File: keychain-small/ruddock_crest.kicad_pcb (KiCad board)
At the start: 2 copper layers, 38 x 45.3 mm, 4 parts

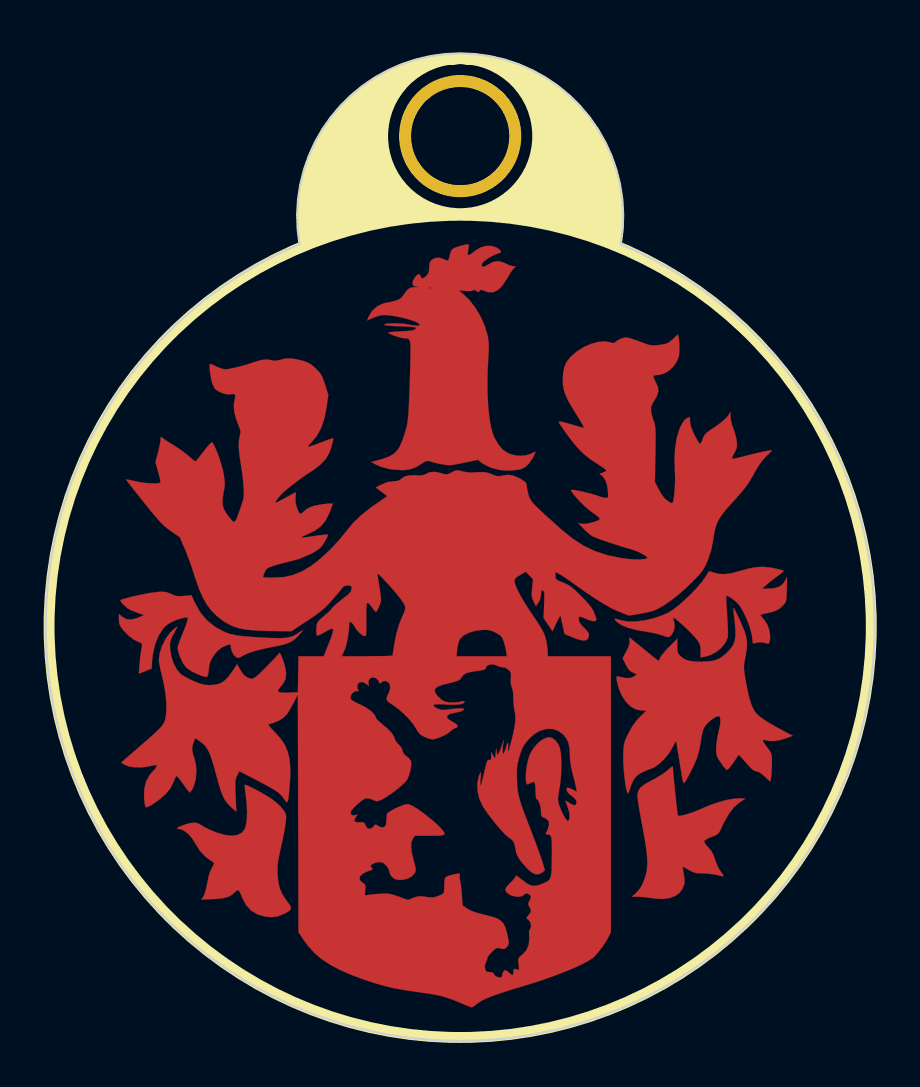
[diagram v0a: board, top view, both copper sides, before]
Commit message: New hole design
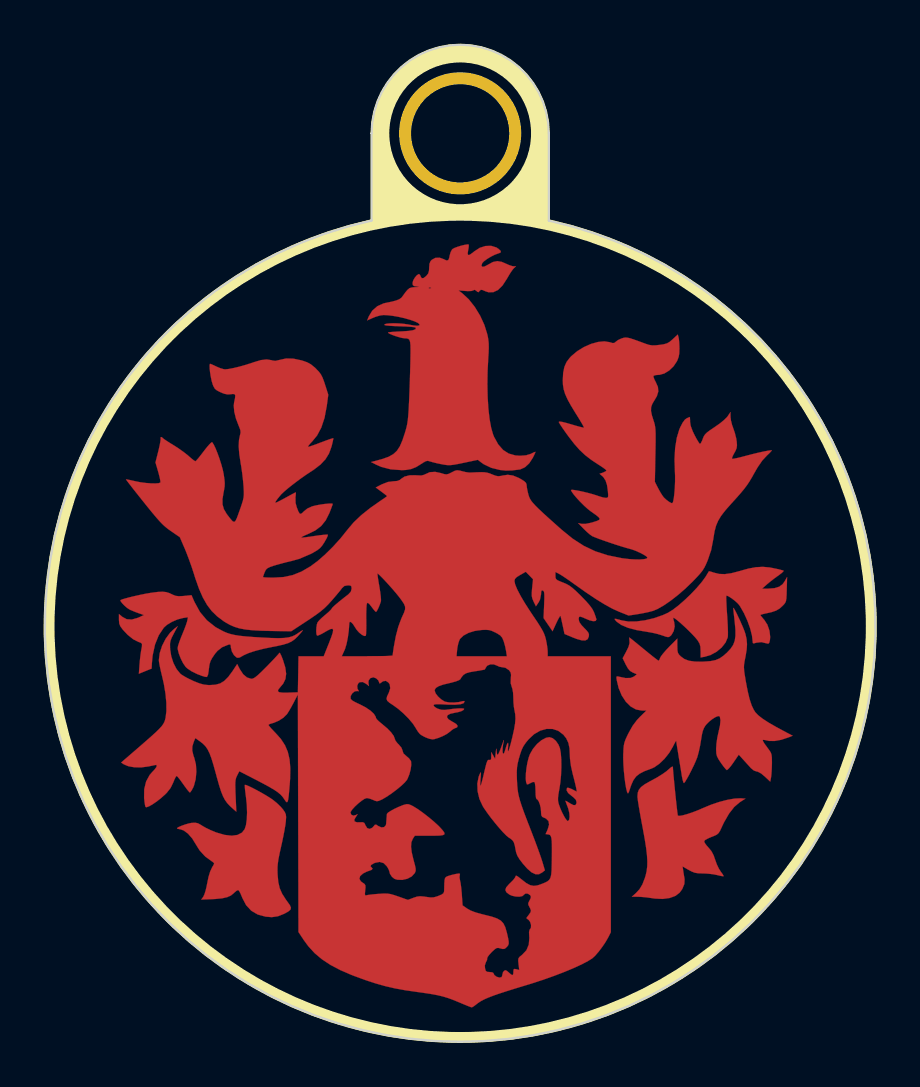
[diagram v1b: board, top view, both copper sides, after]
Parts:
- moved REF** 0.13 mm to (141.0, 85.3)
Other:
- board size 38 x 45.3 mm -> 38.1 x 45.7 mm
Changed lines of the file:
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@@
   (general
     (thickness 1.6)
-    (drawings 22)
+    (drawings 28)
     (tracks 0)
     (zones 0)
@@
   (title_block
     (title "Ruddock House PCB Crest")
-    (date 2019-02-12)
+    (date 2019-02-13)
     (rev A)
     (company "Ruddock House Electrical Engineering")
@@
   )
   (module MountingHole:MountingHole_3.2mm_M3_DIN965_Pad (layer F.Cu)
-    (at 140.97 85.471)
+    (at 140.97 85.344)
     (descr "Mounting Hole 3.2mm, M3, DIN965")
     (tags "mounting hole 3.2mm m3 din965")
@@
       (xy 9.730745 -13.40817) (xy 9.745385 -13.421618) (xy 9.978417 -13.636419) (xy 10.013345 -13.51111)) (layer F.Mask) (width 0.01))
   )
-  (dimension 41.529 (width 0.3) (layer Dwgs.User)
-    (gr_text "41.529 mm" (at 166.946 106.2355 270) (layer Dwgs.User)
+  (gr_poly (pts (xy 144.78 89.408) (xy 141.478 88.9) (xy 143.51 87.884) (xy 144.78 86.106)) (layer B.SilkS) (width 0.15))
+  (gr_poly (pts (xy 144.78 89.408) (xy 141.478 88.9) (xy 143.51 87.884) (xy 144.78 86.106)) (layer F.SilkS) (width 0.15))
+  (gr_poly (pts (xy 137.16 89.408) (xy 140.208 88.9) (xy 138.684 88.138) (xy 137.16 86.106)) (layer B.SilkS) (width 0.15))
+  (gr_poly (pts (xy 137.16 89.408) (xy 140.208 88.9) (xy 138.684 88.138) (xy 137.16 86.106)) (layer F.SilkS) (width 0.15))
+  (gr_line (start 137.16 85.344) (end 137.16 89.408) (layer B.SilkS) (width 0.57))
+  (gr_line (start 144.78 85.344) (end 144.78 89.408) (layer B.SilkS) (width 0.57))
+  (gr_line (start 144.78 85.344) (end 144.78 89.408) (layer F.SilkS) (width 0.57))
+  (gr_arc (start 140.97 85.344) (end 144.78 85.344) (angle -180) (layer B.SilkS) (width 0.57))
+  (gr_circle (center 140.97 85.344) (end 144.47 85.344) (layer B.SilkS) (width 0.5))
+  (gr_line (start 137.16 85.344) (end 137.16 89.408) (layer F.SilkS) (width 0.57))
+  (gr_arc (start 140.97 85.344) (end 144.78 85.344) (angle -180) (layer F.SilkS) (width 0.57))
+  (gr_line (start 145.034 85.344) (end 145.034 89.3445) (layer Edge.Cuts) (width 0.1))
+  (gr_line (start 136.906 85.344) (end 136.906 89.3445) (layer Edge.Cuts) (width 0.1))
+  (gr_arc (start 140.97 107.95) (end 136.906001 89.344501) (angle -335.3568188) (layer Edge.Cuts) (width 0.1))
+  (gr_line (start 121.92 107.95) (end 160.02 107.95) (layer Dwgs.User) (width 0.1))
+  (gr_arc (start 140.97 85.344) (end 145.034 85.344) (angle -180) (layer Edge.Cuts) (width 0.1))
+  (gr_circle (center 140.97 85.344) (end 144.47 85.344) (layer F.SilkS) (width 0.5))
+  (gr_line (start 140.97 128.27) (end 140.97 78.74) (layer Dwgs.User) (width 0.1))
+  (dimension 38.1 (width 0.3) (layer Dwgs.User)
+    (gr_text "38.100 mm" (at 140.97 134.179999) (layer Dwgs.User)
       (effects (font (size 1.5 1.5) (thickness 0.3)))
     )
-    (feature1 (pts (xy 149.098 127) (xy 165.432421 127)))
-    (feature2 (pts (xy 149.098 85.471) (xy 165.432421 85.471)))
-    (crossbar (pts (xy 164.846 85.471) (xy 164.846 127)))
-    (arrow1a (pts (xy 164.846 127) (xy 164.259579 125.873496)))
-    (arrow1b (pts (xy 164.846 127) (xy 165.432421 125.873496)))
-    (arrow2a (pts (xy 164.846 85.471) (xy 164.259579 86.597504)))
-    (arrow2b (pts (xy 164.846 85.471) (xy 165.432421 86.597504)))
+    (feature1 (pts (xy 160.02 128.27) (xy 160.02 132.66642)))
+    (feature2 (pts (xy 121.92 128.27) (xy 121.92 132.66642)))
+    (crossbar (pts (xy 121.92 132.079999) (xy 160.02 132.079999)))
+    (arrow1a (pts (xy 160.02 132.079999) (xy 158.893496 132.66642)))
+    (arrow1b (pts (xy 160.02 132.079999) (xy 158.893496 131.493578)))
+    (arrow2a (pts (xy 121.92 132.079999) (xy 123.046504 132.66642)))
+    (arrow2b (pts (xy 121.92 132.079999) (xy 123.046504 131.493578)))
   )
-  (dimension 45.339044 (width 0.3) (layer Dwgs.User)
-    (gr_text "45.339 mm" (at 171.767588 104.290968 270.0802461) (layer Dwgs.User)
-      (effects (font (size 1.5 1.5) (thickness 0.3)))
-    )
-    (feature1 (pts (xy 143.5735 127) (xy 170.285761 126.962588)))
-    (feature2 (pts (xy 143.51 81.661) (xy 170.222261 81.623588)))
-    (crossbar (pts (xy 169.63584 81.624409) (xy 169.69934 126.963409)))
-    (arrow1a (pts (xy 169.69934 126.963409) (xy 169.111342 125.837728)))
-    (arrow1b (pts (xy 169.69934 126.963409) (xy 170.284182 125.836085)))
-    (arrow2a (pts (xy 169.63584 81.624409) (xy 169.050998 82.751733)))
-    (arrow2b (pts (xy 169.63584 81.624409) (xy 170.223838 82.75009)))
-  )
-  (gr_line (start 138.43 85.471) (end 143.51 85.471) (layer Dwgs.User) (width 0.1))
-  (gr_poly (pts (xy 148.082 90.424) (xy 141.986 88.9) (xy 144.272 87.376) (xy 144.526 84.328) (xy 143.256 82.296) (xy 146.558 84.328) (xy 148.082 87.63)) (layer B.SilkS) (width 0.15))
-  (gr_poly (pts (xy 148.082 90.424) (xy 141.986 88.9) (xy 144.272 87.376) (xy 144.526 84.328) (xy 143.256 82.296) (xy 146.558 84.328) (xy 148.082 87.63)) (layer F.SilkS) (width 0.15))
-  (gr_poly (pts (xy 133.858 90.424) (xy 139.954 88.9) (xy 137.668 87.376) (xy 137.414 84.328) (xy 138.938 82.042) (xy 135.128 84.582) (xy 133.858 87.63)) (layer B.SilkS) (width 0.15))
-  (gr_poly (pts (xy 133.858 90.424) (xy 139.954 88.9) (xy 137.668 87.376) (xy 137.414 84.328) (xy 138.938 82.042) (xy 135.128 84.582) (xy 133.858 87.63)) (layer F.SilkS) (width 0.15))
-  (gr_arc (start 140.97 89.145) (end 148.081999 90.437999) (angle -200.2) (layer B.SilkS) (width 0.5))
-  (gr_arc (start 140.97 89.145) (end 148.081999 90.437999) (angle -200.2) (layer F.SilkS) (width 0.5))
-  (gr_circle (center 140.97 85.471) (end 144.526 85.471) (layer B.SilkS) (width 0.5))
-  (gr_arc (start 140.97 89.14) (end 148.081999 90.423999) (angle -200.2) (layer F.SilkS) (width 0.5))
+  (gr_line (start 121.92 88.9) (end 121.92 127) (layer Dwgs.User) (width 0.1))
+  (gr_line (start 160.02 88.9) (end 121.92 88.9) (layer Dwgs.User) (width 0.1))
+  (gr_line (start 160.02 127) (end 160.02 88.9) (layer Dwgs.User) (width 0.1))
+  (gr_line (start 121.92 127) (end 160.02 127) (layer Dwgs.User) (width 0.1))
+  (gr_line (start 136.398 85.344) (end 145.542 85.344) (layer Dwgs.User) (width 0.1))
   (gr_line (start 140.716 89.154) (end 141.224 89.154) (layer Dwgs.User) (width 0.1))
-  (gr_line (start 140.97 78.74) (end 140.97 129.54) (layer Dwgs.User) (width 0.1))
-  (gr_arc (start 140.97 89.154) (end 148.335999 90.423999) (angle -199.5648141) (layer Edge.Cuts) (width 0.1))
-  (gr_line (start 149.352 90.424) (end 133.096 90.424) (layer Dwgs.User) (width 0.1))
-  (gr_arc (start 140.97 107.95) (end 133.604001 90.424001) (angle -314.4) (layer Edge.Cuts) (width 0.1))
-  (gr_circle (center 140.97 85.471) (end 144.526 85.471) (layer F.SilkS) (width 0.5))
   (gr_circle (center 140.97 107.95) (end 159.82 107.95) (layer B.SilkS) (width 0.5))
   (gr_circle (center 140.97 107.95) (end 159.82 107.95) (layer F.SilkS) (width 0.5))
-  (gr_circle (center 140.97 107.95) (end 139.7 107.95) (layer Dwgs.User) (width 0.1))
-  (dimension 38.1 (width 0.3) (layer Dwgs.User)
-    (gr_text "38.100 mm" (at 140.97 134.18) (layer Dwgs.User)
-      (effects (font (size 1.5 1.5) (thickness 0.3)))
-    )
-    (feature1 (pts (xy 160.02 111.76) (xy 160.02 132.666421)))
-    (feature2 (pts (xy 121.92 111.76) (xy 121.92 132.666421)))
-    (crossbar (pts (xy 121.92 132.08) (xy 160.02 132.08)))
-    (arrow1a (pts (xy 160.02 132.08) (xy 158.893496 132.666421)))
-    (arrow1b (pts (xy 160.02 132.08) (xy 158.893496 131.493579)))
-    (arrow2a (pts (xy 121.92 132.08) (xy 123.046504 132.666421)))
-    (arrow2b (pts (xy 121.92 132.08) (xy 123.046504 131.493579)))
-  )
   (gr_circle (center 140.97 107.95) (end 140.97 88.9) (layer Dwgs.User) (width 0.1))
 )
